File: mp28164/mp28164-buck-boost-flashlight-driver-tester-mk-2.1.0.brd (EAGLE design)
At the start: 20 x 15 mm, 23 parts, among them J1 AVR_SPI_PRG_6PTH, U1 MPS28164, U2 ATTINY1310M1, U3 LMP8646, U4 V_REG_ENTLV700

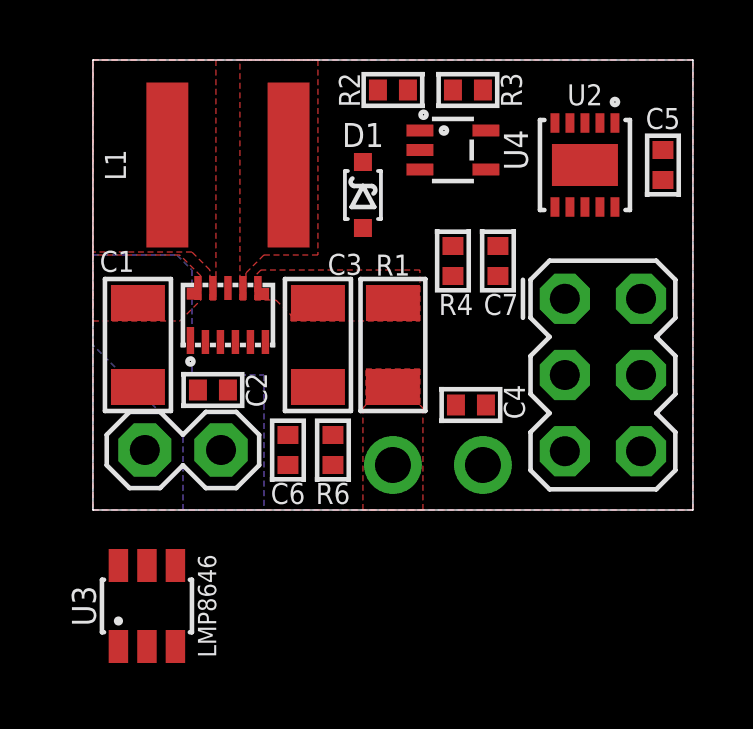
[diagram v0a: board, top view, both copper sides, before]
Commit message: wip buck boost
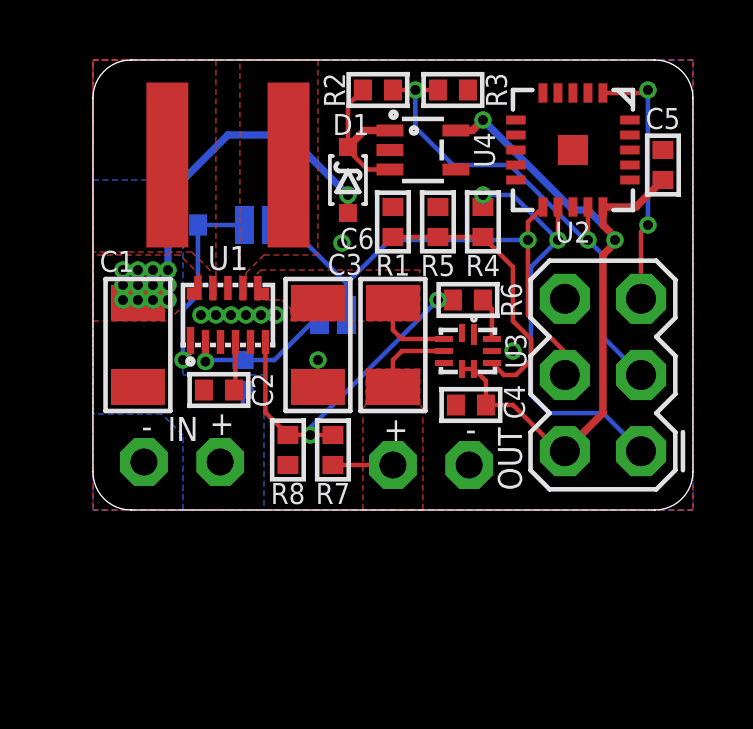
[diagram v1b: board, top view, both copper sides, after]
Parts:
- removed +, -: M01PTH-1.2MM-NS, a_parts:1X01-1.2MM-NS
- removed C7: 1nF, a_parts:C0402
- added EN, MODE: JUMPER-PAD-2-NOYES_SILK, a_parts:PAD-JUMPER-2-NO_YES_SILK
- added JP2: M021X02_NO_SILK, a_parts:1X02_NO_SILK
- added R10, R9: DNP, a_parts:R0402
- added R5: 220R, a_parts:R0402
- added R7: 560K, a_parts:R0402
- added R8: 100K, a_parts:R0402
- C6: value 1nF -> 10nF
- JP1: value M02PTH-CENTERED -> M021X02_NO_SILK; device a_parts:1X02-CENTER -> a_parts:1X02_NO_SILK
- R4: value 6.8k -> 1.02K
- R6: value 6.8k -> 0R
- U2: value ATTINY1310M1 -> ATTINY25-20MU; device a_parts:QFN10(2X5) -> a_parts:QFN20
- U3: value LMP8646 -> INA190RSW; device a_parts:SOT23-6 -> a_parts:UQFN-10
- U4: value V_REG_ENTLV700 -> TLV30028DCK
- moved U3 13.7 mm to (12.5, 5.30), turned to 180 degrees
- moved C6 8.37 mm to (10.0, 9.60), turned to 90 degrees
- moved R6 6.73 mm to (12.5, 7.00), turned to 0 degrees
- moved R4 1.64 mm to (13.0, 9.60)
- moved JP1 1.36 mm to (1.70, 1.60)
- moved U4 1.00 mm to (11.0, 12.0)
- moved D1 0.71 mm to (8.50, 11.0)
- moved U2 0.64 mm to (16.0, 12.0)
- moved R2 0.50 mm to (9.50, 14.0)
- moved R3 0.50 mm to (12.0, 14.0)
- moved C2 0.20 mm to (4.20, 4.00)
- turned J1 to 90 degrees
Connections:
- new net EN: EN.2, R9.2, U1.1
- new net MODE/SYNC: MODE.2, R10.2, U1.2
- net ALTPWM/MOSI: now also EN.1, MODE.1, U2.11; no longer U1.2, U2.6
- net CSOUT: now also U3.10
- net FB: now also R7.2, R8.2; no longer C6.1
- net GND: now also JP2.1, R5.2, R8.1, U2.8, U3.9; no longer -.P$1, C7.1, U2.5, U3.2
- net LED+: now also JP2.2, R7.1; no longer +.P$1
- net PWM/MISO: now also U2.12; no longer C7.2, U2.7
- net REF: now also C6.1, R5.1, U3.8
- net VBAT: now also R10.1, R9.1; no longer U1.1
- net VCC: now also U2.15, U3.7; no longer U2.10
- net VDIV/SCK: now also U2.14; no longer U2.9
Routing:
- net VCC: track 0.00 -> 23.6 mm, vias 0 -> 2
- net ALTPWM/MOSI: track 0.00 -> 17.3 mm, vias 0 -> 1
- net VDIV/SCK: track 0.00 -> 16.4 mm, vias 0 -> 2
- net PWM/MISO: track 0.00 -> 14.6 mm, vias 0 -> 2
- net FB: track 0.00 -> 11.7 mm, vias 0 -> 2
- net VBAT: track 0.00 -> 11.3 mm, vias 0 -> 13
- net REF: track 0.00 -> 9.44 mm
- net RST: track 0.00 -> 8.60 mm, vias 0 -> 2
- net EN: track 0.00 -> 7.01 mm, vias 0 -> 1
- net VBAT_RECT: track 0.00 -> 5.50 mm
- net MODE/SYNC: track 0.00 -> 5.25 mm, vias 0 -> 1
- net LED+: track 0.00 -> 4.72 mm
- net VOUT: track 0.00 -> 2.72 mm
- net VDD: track 0.00 -> 1.62 mm
- net CSOUT: track 0.00 -> 1.42 mm
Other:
- outline, holes or cut-outs redrawn
- board text added: "+"
- board text added: "-"
- board text added: "IN"
- board text added: "OUT"
